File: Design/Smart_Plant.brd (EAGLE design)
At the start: 80 x 129.1 mm, 70 parts, among them IC1 TP4056, IC2 TLC555CDR, IC3 AHT20, IC4 RT9080-33GJ5, IC5 ESP32-S3-MINI-1-N8, J6 USB-C, Q1 IRLML0100, Q2 ALS-PT19-315C, T1 MMBT2222A, T2 LBSS84LT1G, U1 ESP-32S

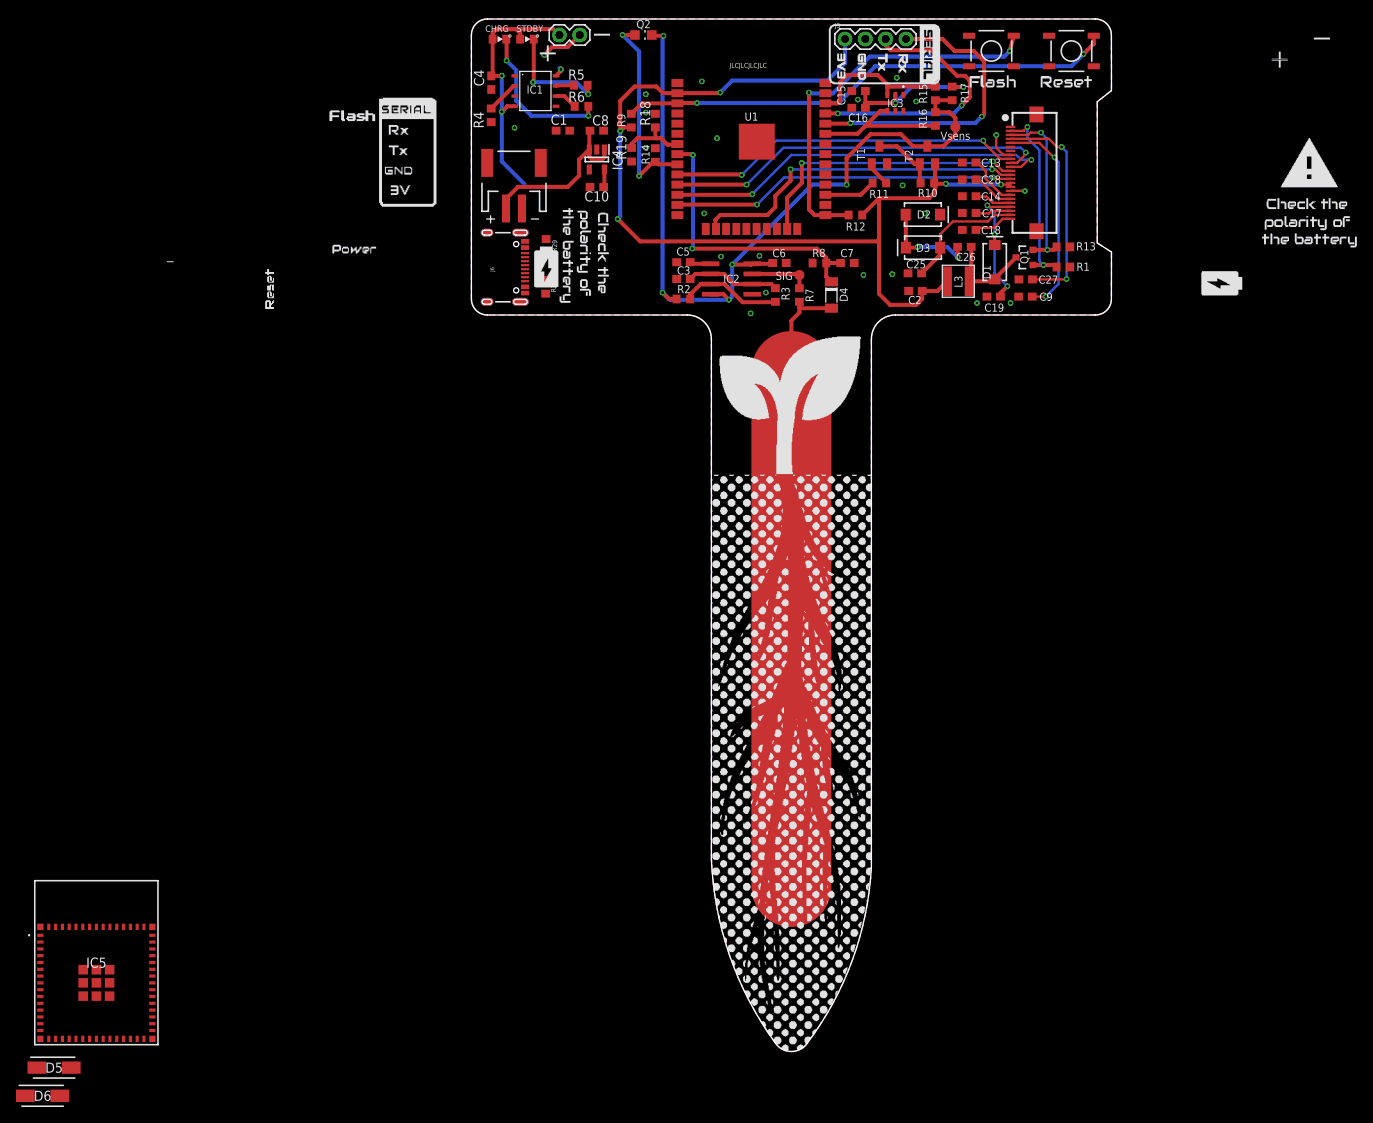
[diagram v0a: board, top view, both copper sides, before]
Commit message: Released designs from V1R1 with the patch board
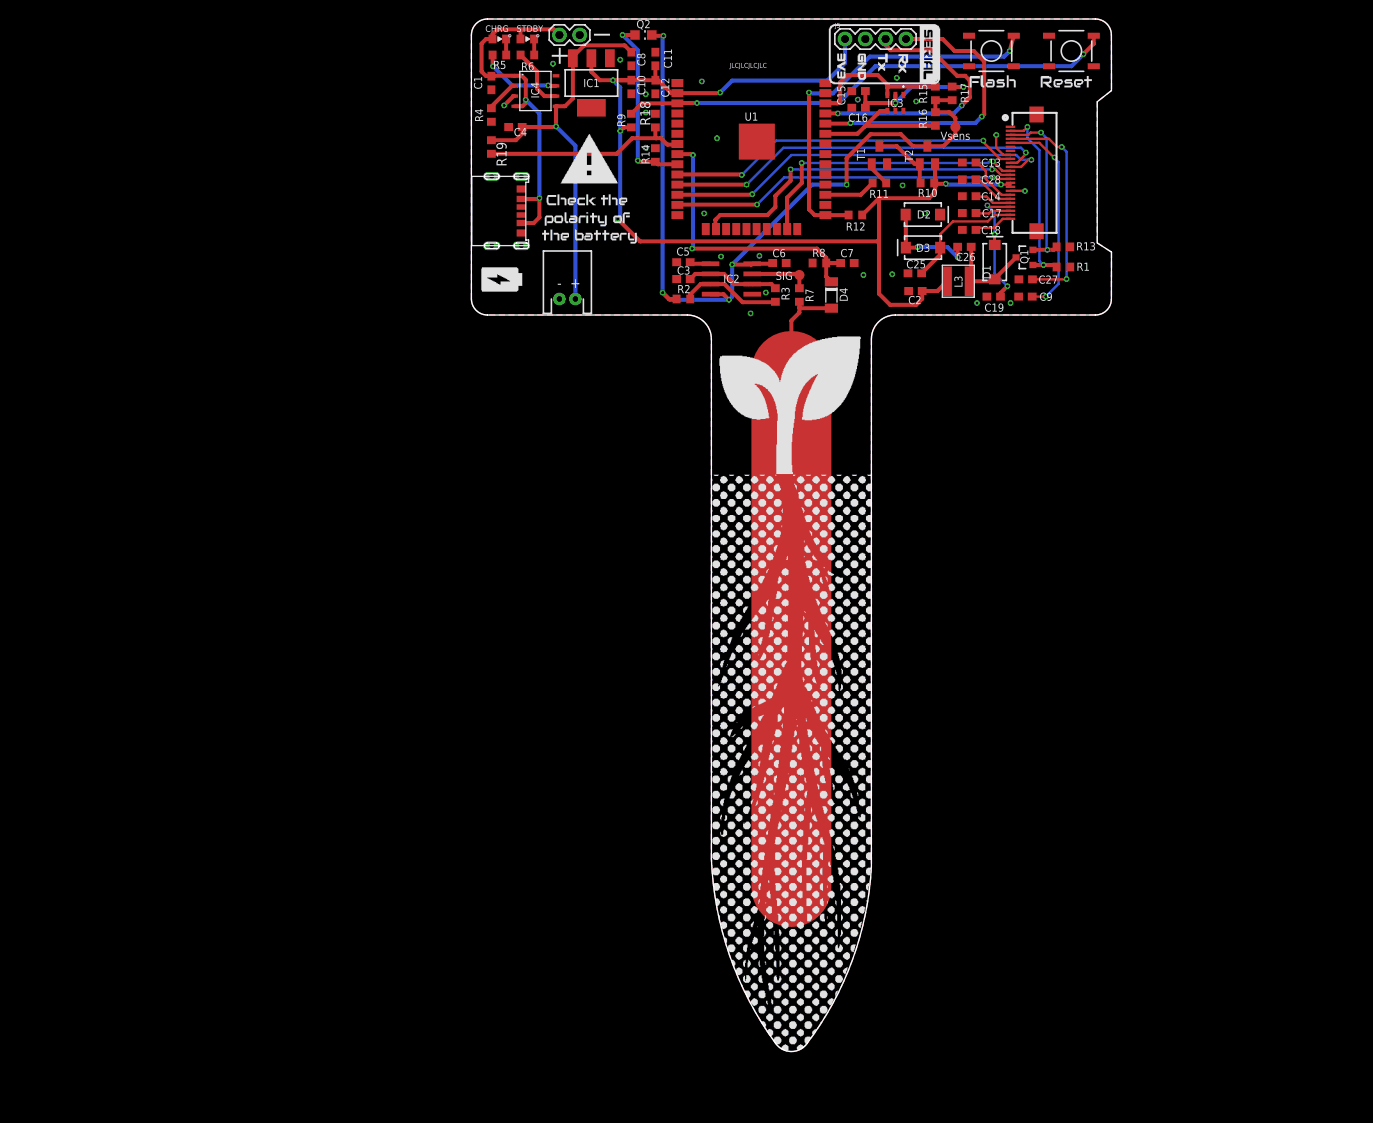
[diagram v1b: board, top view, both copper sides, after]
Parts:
- removed D5, D6: B340A-13-F, SamacSys_Parts:DIOM5226X240N
- removed IC5: ESP32-S3-MINI-1-N8, SamacSys_Parts:ESP32S3MINI1N8
- removed J6: USB-C, SparkFun-Connectors:USB-C-16P-4LAYER-ISOLATED
- removed R28, R29: 5.1k, rcl:R0603
- added C11: 100nF, rcl:C0603
- added C12: 22uF, rcl:C0603
- added J2: USBC-6P, SpaceDIY_connectors:USCX-06FX-XXMX-01
- IC1: value TP4056 -> AMS1117-3.3; device TP4056:SOT23-8 -> SparkFun-IC-Power:SOT223
- IC4: value RT9080-33GJ5 -> TP4056; device SamacSys_Parts:SOT94P280X100-5N -> TP4056:SOT23-8
- J4: device SpaceDIY_connectors:JST-2-SMD -> SparkFun-Connectors:JST-2-PTH-NS
- moved R19 17.5 mm to (2.50, 21.0), turned to 270 degrees
- moved J4 16.7 mm to (12.0, 2.00), turned to 0 degrees
- moved C10 13.2 mm to (20.0, 28.5), turned to 270 degrees
- moved IC4 11.5 mm to (8.00, 28.0)
- moved R5 10.9 mm to (3.50, 32.5)
- moved C1 10.7 mm to (2.50, 29.0), turned to 270 degrees
- moved C8 9.95 mm to (20.0, 32.0), turned to 270 degrees
- moved R6 9.32 mm to (7.00, 32.5)
- moved IC1 7.07 mm to (15.0, 29.0), turned to 180 degrees
- moved C4 6.31 mm to (5.50, 23.5), turned to 180 degrees
- moved LED2 3.48 mm to (7.00, 34.5)
- moved LED1 3.46 mm to (3.50, 34.5)
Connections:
- removed net CC1: J6.B5, R28.2
- removed net CC2: J6.A5, R29.2
- removed net D+: J6.A6, J6.B6
- removed net D-: J6.A7, J6.B7
- removed net N$35: D6.2, J1.1
- removed net N$4 (its old number): IC1.2, R4.2
- removed net V_USB: D5.2, J6.VBUS1, J6.VBUS2
- new net N$2: IC4.6, R6.2
- net 3.3V: now also C11.1, C12.1, IC1.2; no longer IC4.5, IC5.3
- net BATTERY: no longer IC5.31
- net GND: now also C11.2, C12.2, IC4.3, IC4.8, J2.GND1, J2.GND2, J4.1; no longer IC1.3, IC4.2, IC5.1, IC5.2, IC5.42, IC5.43, IC5.46, IC5.47, IC5.48, IC5.49, IC5.50, IC5.51, IC5.52, IC5.53, IC5.54, IC5.55, IC5.56, IC5.57, IC5.58, IC5.59, IC5.60, IC5.61, IC5.62, IC5.63, IC5.64, IC5.65, IC5.66, IC5.67, IC5.68, IC5.69, IC5.70, IC5.71, IC5.72, IC5.73, J4.2, J6.GND, J6.GND2, R28.1, R29.1
- net N$1: now also IC4.2, R4.2; no longer IC1.6, R6.2
- net N$6: now also IC4.7; no longer IC1.7
- net RST: no longer IC5.45
- net VBAT: now also C4.1, IC1.3, IC4.5, J4.2; no longer C1.1, IC1.5, IC4.1, IC4.3, J4.1
- net VIN: now also C1.1, IC4.1, IC4.4, J1.1, J2.VBUS1, J2.VBUS2; no longer C4.1, D5.1, D6.1, IC1.4, IC1.8
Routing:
- net VBAT: track 21.8 -> 50.4 mm, vias 0 -> 1
- net BATTERY: track 8.27 -> 25.8 mm
- net N$4: track 19.2 -> 2.00 mm, vias 2 -> 0
- net VIN: track 34.7 -> 46.9 mm, vias 3 -> 2
- net N$3: track 14.1 -> 2.00 mm, vias 2 -> 0
- net 3.3V: track 133.2 -> 142.9 mm, vias 5 -> 6
- net N$6: track 2.29 -> 10.3 mm, vias 0 -> 2
- net N$2: track 0.00 -> 7.82 mm
- net N$4 (its old number): track 4.11 -> 0.00 mm
- net GND: track 11.0 -> 7.38 mm, vias 23 -> 24
- net LIGHT: track 25.7 -> 23.2 mm
- net N$1: track 2.86 -> 4.19 mm
